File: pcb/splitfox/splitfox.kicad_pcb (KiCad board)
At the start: 2 copper layers, 255.8 x 122.5 mm, 137 parts, among them CN1 S7B-ZR-SM4A-TF(LF)(SN)_C51187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, CN2 S7B-ZR-SM4A-TF(LF)(SN)_C51187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, SW1 TS24CA, SW2 SS-12D07-L5-B, SW3 GT-TC152A-H085-L1, SW4 GT-TC152A-H085-L1, SW5 GT-TC152A-H085-L1, SW6 GT-TC152A-H085-L1, SW7 GT-TC152A-H085-L1, SW8 GT-TC152A-H085-L1, U1 RP2040, U2 SN74LV1T34DBVR, U3 W25Q128JVS, U4 XC6206PxxxMR-Regulator_Linear, U5 USBLC6-2SC6, Y1 12MHz

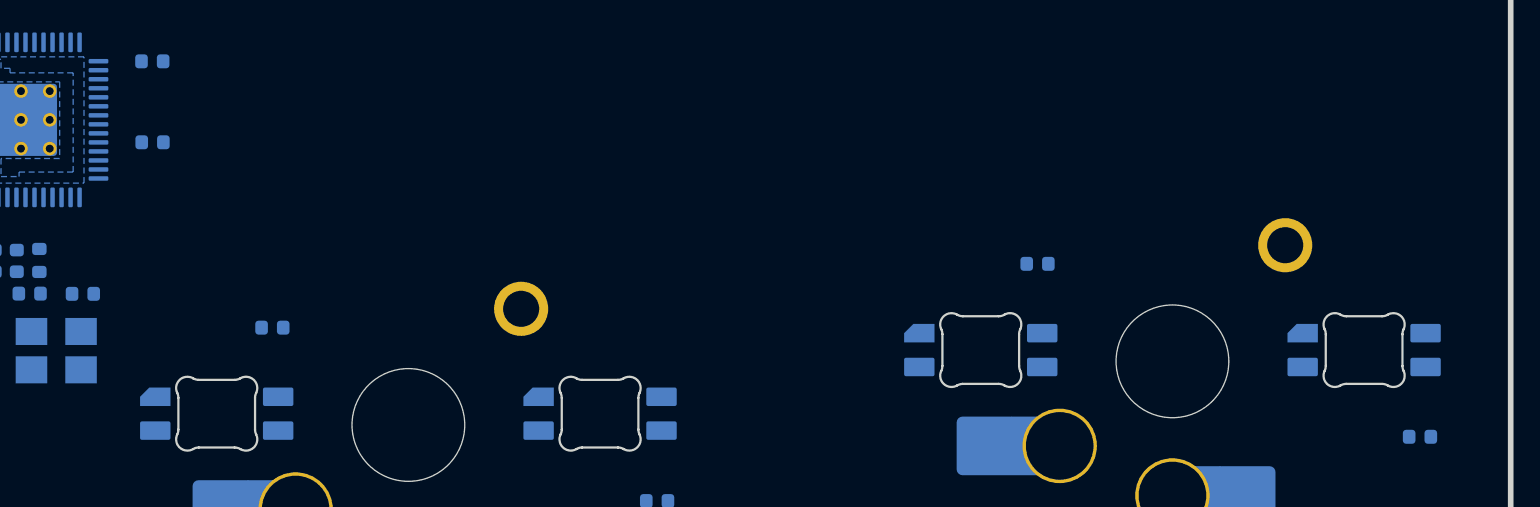
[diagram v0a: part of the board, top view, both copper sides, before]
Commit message: NG | Ready for routing
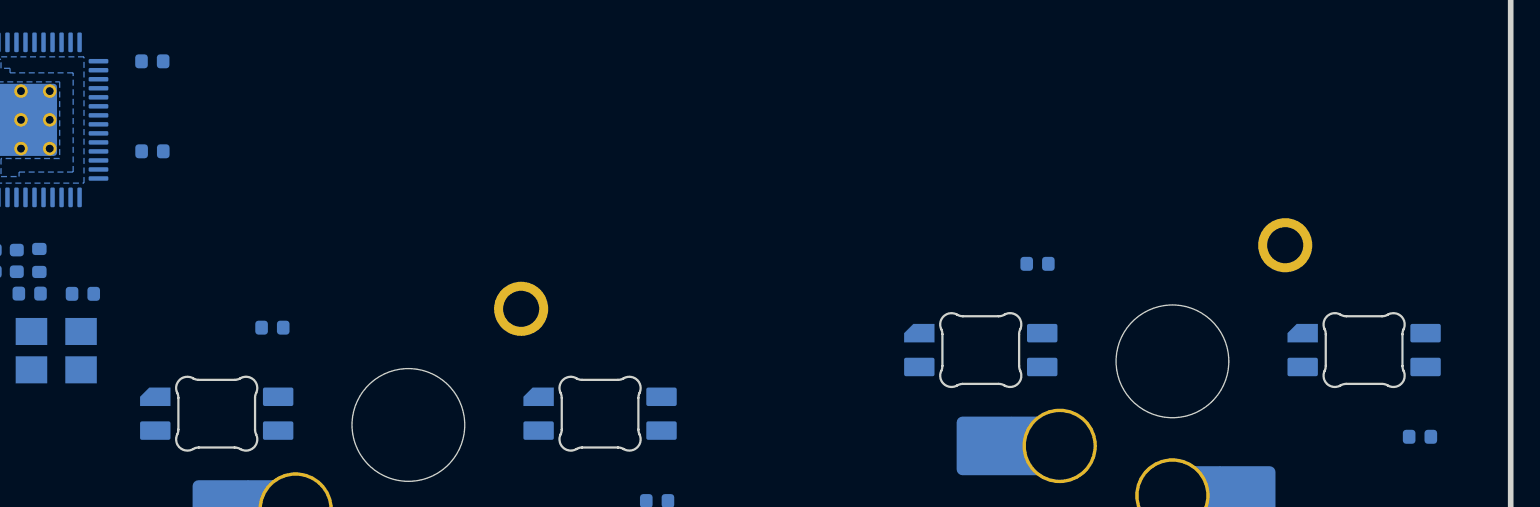
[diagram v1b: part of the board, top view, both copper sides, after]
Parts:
- moved C20 0.40 mm to (154.1, 124.7)
